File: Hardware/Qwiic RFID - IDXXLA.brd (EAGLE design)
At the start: 25.4 x 30.5 mm, 60 parts, among them J2 SMD, J3 PTH, J4 SMD, J8 AVR_SPI_PROG_3X2TESTPOINTS, Q1 600mA/40V, U1 ATTINY84-ARDUINO, U2 ID-12/20SMD

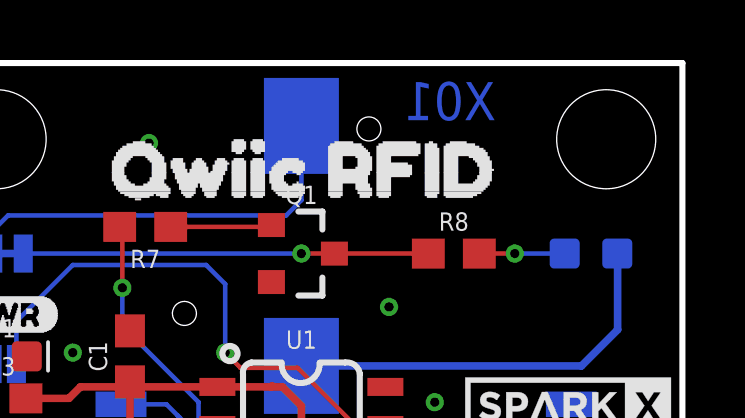
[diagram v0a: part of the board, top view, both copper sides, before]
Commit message: Panel for x02
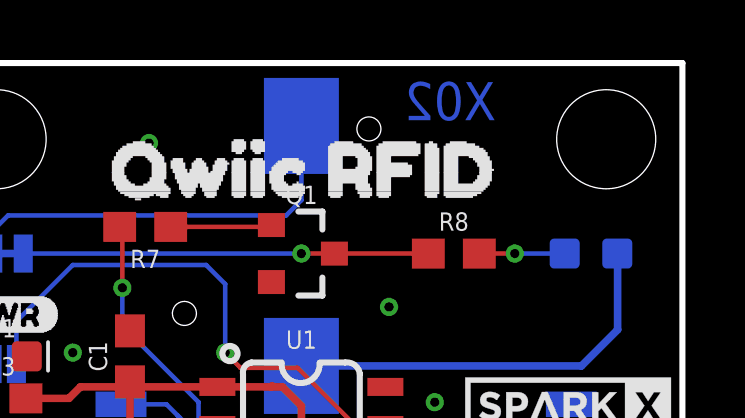
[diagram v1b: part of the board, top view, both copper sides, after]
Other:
- board text added: "X02"
- board text removed: "X01"
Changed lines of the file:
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@@
 <wire x1="25.4" y1="30.48" x2="25.4" y2="0" width="0.2032" layer="20"/>
 <wire x1="25.4" y1="0" x2="0" y2="0" width="0.2032" layer="20"/>
-<text x="17.653" y="29.21" size="1.27" layer="16" font="vector" ratio="15" rot="MR0" align="center">X01</text>
+<text x="17.653" y="29.21" size="1.27" layer="16" font="vector" ratio="15" rot="MR0" align="center">X02</text>
 <text x="1.27" y="38.1" size="1.778" layer="47" font="vector" ratio="15">Units in Inches</text>
 <text x="21.59" y="-10.16" size="1.778" layer="51" font="vector" ratio="15">Elias Santistevan</text>
